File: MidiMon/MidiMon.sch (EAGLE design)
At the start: 55 parts, among them IC1 PIC18F4520-I/P, IC2 6N138, IC5 7805TV, J1 DIN5, J2 DIN5, J4 2.1MMJACKTHM, X1 ECS-100-18-4X

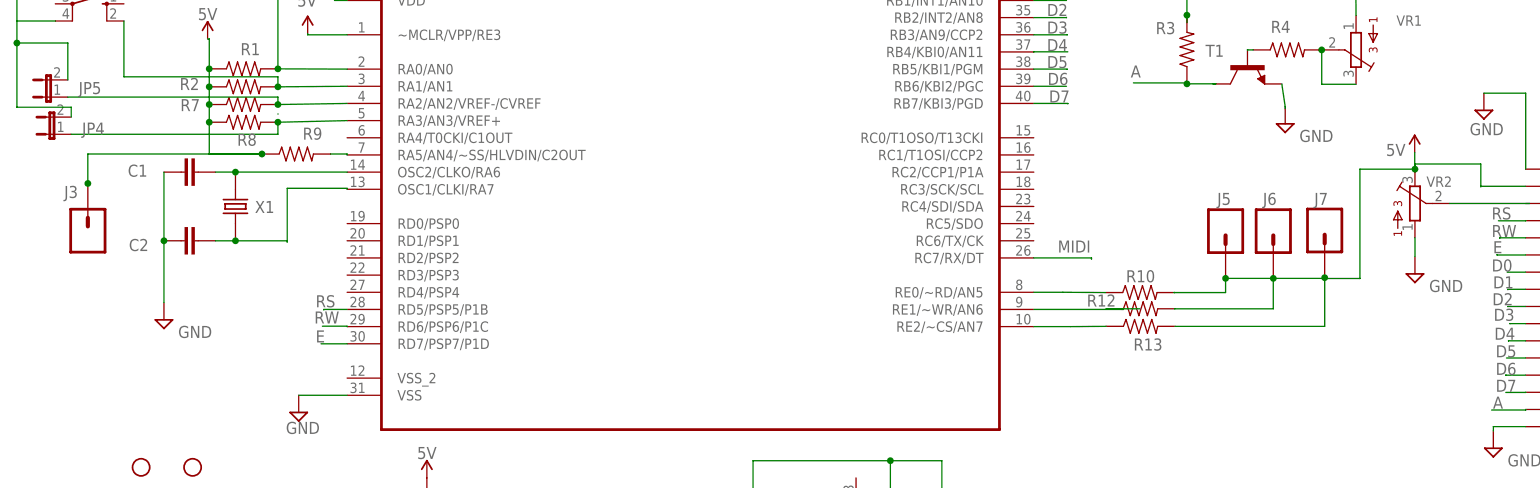
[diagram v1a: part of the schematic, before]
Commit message: Adjustments made Signed-off-by: goslo <digit99@mailinator.com>
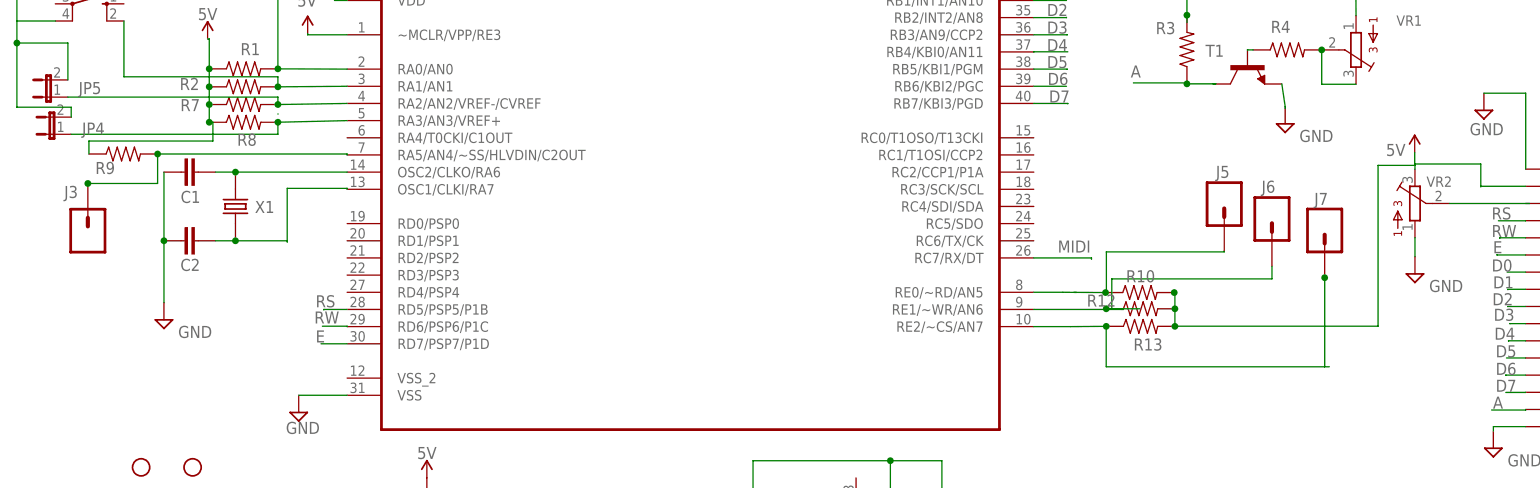
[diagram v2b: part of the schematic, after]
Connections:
- removed net N$8: IC1.RA5/AN4/~SS/HLVDIN/C2OUT, R9.2
- new net N$20: IC1.RA5/AN4/~SS/HLVDIN/C2OUT, J3.1, R9.2
- net 5V: now also R10.2, R12.2, R13.2; no longer J3.1
- net N$18: no longer J5.1, J6.1, J7.1, R10.2, R12.2, R13.2
- net N$29: now also J6.1
- net N$30: now also J5.1
- net N$31: now also J7.1
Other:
- moved on the sheet: J5, J6, R9
